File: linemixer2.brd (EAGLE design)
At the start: 101.6 x 58.4 mm, 75 parts, among them IC1 OPA2134P, IC2 OPA2134P, IC3 OPA2134P, IC4 OPA2134P, IC5 OPA2134P, IC6 BUF634P, J1 POWER_JACK

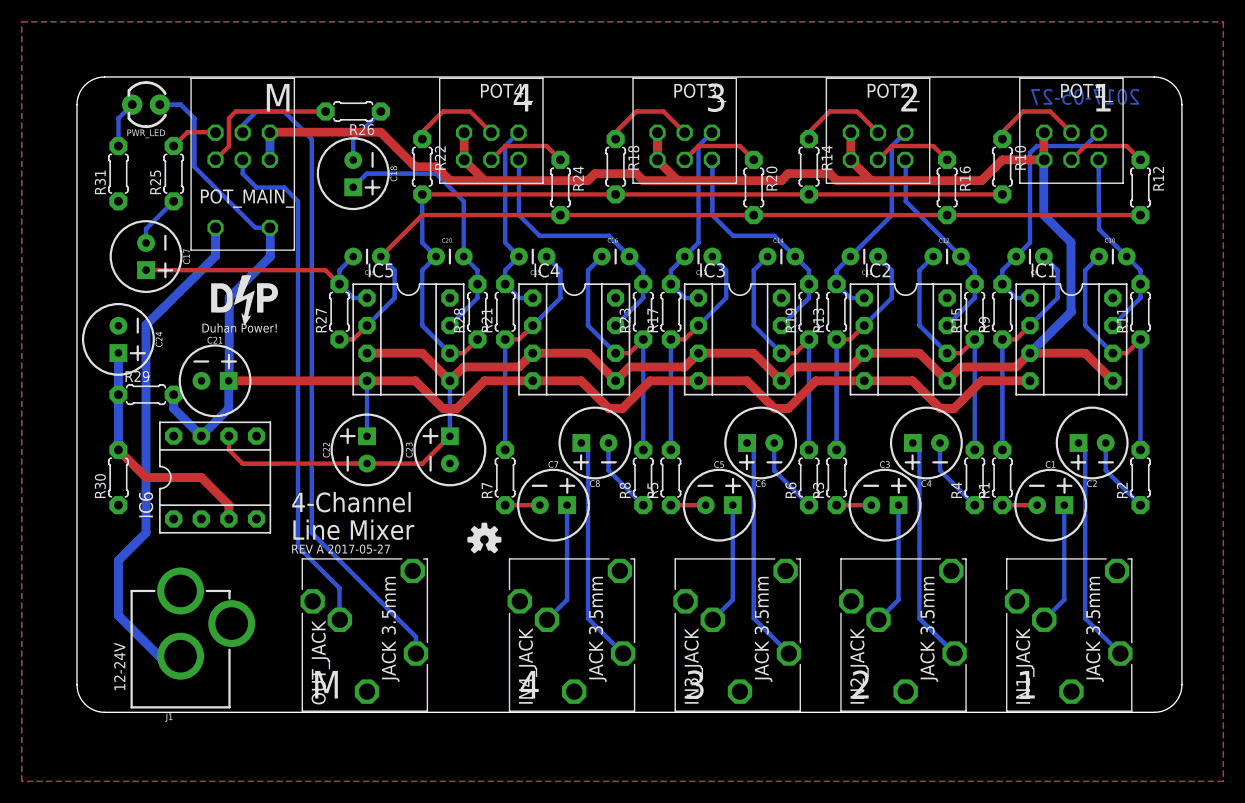
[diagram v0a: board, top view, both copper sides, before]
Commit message: rev b
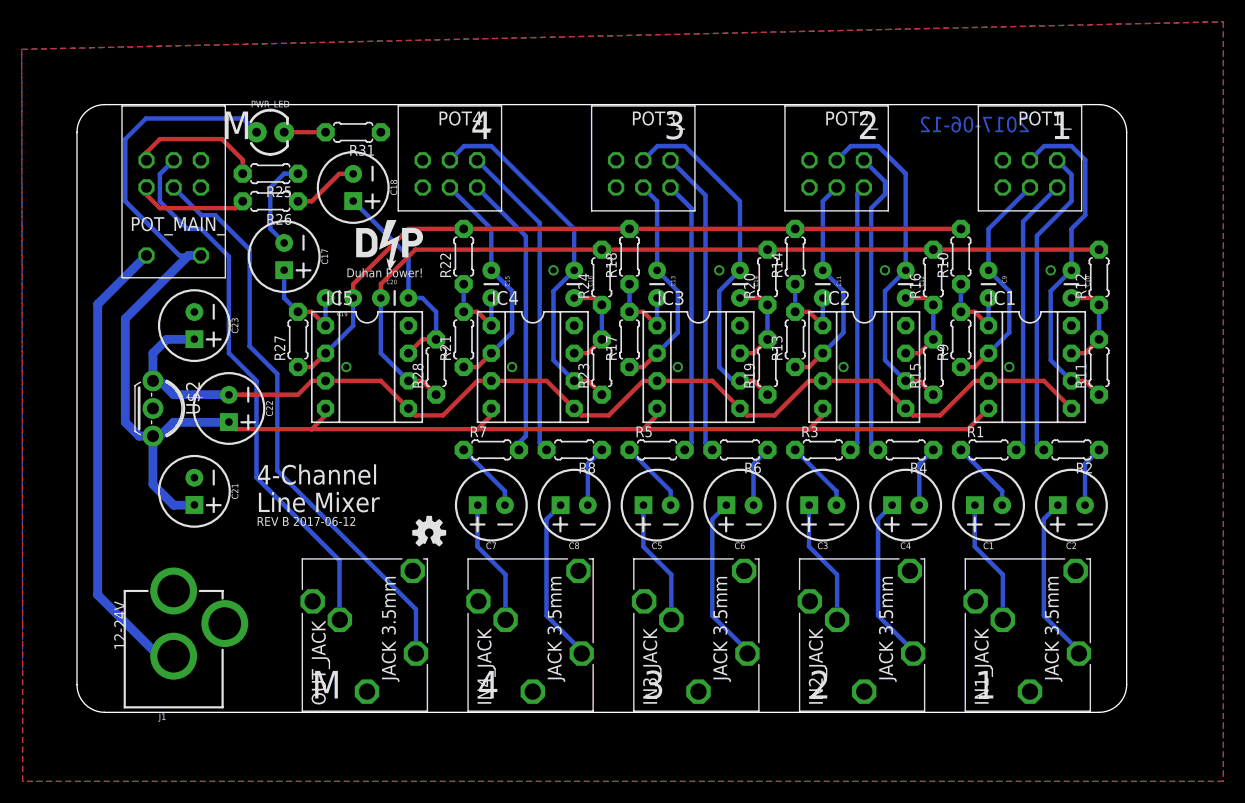
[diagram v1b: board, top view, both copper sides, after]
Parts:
- removed C24: 47u, SparkFun-Capacitors:CPOL-RADIAL-2.5MM-6.5MM
- removed IC6: BUF634P, burr-brown:DIL08
- removed R29, R30: 10k, adafruit:0204/5
- added U$2: TLE2426-TO_92, myparts:TO-92
- R1, R2, R3, R4, R5, R6, R7, R8: value 10k -> 1k
- R10, R12, R14, R16, R18, R20, R22, R24: value 22k -> 1k
- R11, R13, R15, R17, R19, R21, R23, R27, R28, R9: value 47k -> 1k
- R31: value 1k -> 5k
- moved C23 26.1 mm to (10.8, 35.6), turned to 270 degrees
- moved R31 21.9 mm to (25.4, 53.3), turned to 180 degrees
- moved U$1 14.3 mm to (28.6, 43.2)
- moved C22 13.3 mm to (14.0, 27.9), turned to 270 degrees
- moved C17 12.7 mm to (19.1, 41.9)
- moved PWR_LED 11.7 mm to (17.8, 53.3), turned to 0 degrees
- moved R26 11.2 mm to (17.8, 47.0)
- moved C21 10.3 mm to (10.8, 20.3), turned to 270 degrees
- moved R10 9.09 mm to (81.3, 41.9), turned to 90 degrees
- moved R22 9.09 mm to (35.6, 41.9), turned to 90 degrees
- moved R12 9.09 mm to (94.0, 40.0), turned to 90 degrees
- moved R24 9.09 mm to (48.3, 40.0), turned to 90 degrees
- moved R25 8.89 mm to (17.8, 49.5), turned to 180 degrees
- moved R14 8.35 mm to (66.0, 41.9), turned to 90 degrees
- moved R18 8.35 mm to (50.8, 41.9), turned to 90 degrees
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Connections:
- removed net N$19: POT1_.R1-W, R10.1
- removed net N$20: POT2_.R1-W, R14.1
- removed net N$24: POT1_.R2-W, R12.1
- removed net N$26: POT2_.R2-W, R16.1
- removed net N$28: POT3_.R1-W, R18.1
- removed net N$30: POT3_.R2-W, R20.1
- removed net N$32: POT4_.R1-W, R22.1
- removed net N$34: POT4_.R2-W, R24.1
- removed net N$44: C24.1, IC6.3, R29.1, R30.2
- new net N$40: C9.1, IC1.2, POT1_.R2-W, R9.1
- new net N$50: C13.1, IC3.2, POT3_.R2-W, R17.1
- new net N$51: C11.1, IC2.2, POT2_.R2-W, R13.1
- new net N$52: C15.1, IC4.2, POT4_.R2-W, R21.1
- new net N$60: C10.1, IC1.6, POT1_.R1-W, R11.1
- new net N$61: C12.1, IC2.6, POT2_.R1-W, R15.1
- new net N$62: C14.1, IC3.6, POT3_.R1-W, R19.1
- new net N$64: C16.1, IC4.6, POT4_.R1-W, R23.1
- net BUS_L: now also R10.2, R14.2, R18.2, R22.2; no longer R12.2, R16.2, R20.2, R24.2
- net BUS_R: now also R12.2, R16.2, R20.2, R24.2; no longer R10.2, R14.2, R18.2, R22.2
- net GND: now also POT1_.R1-A, POT1_.R2-A, POT2_.R1-A, POT2_.R2-A, POT3_.R1-A, POT3_.R2-A, POT4_.R1-A, POT4_.R2-A, POT_MAIN_.R1-A, POT_MAIN_.R2-A, U$2.PAD2; no longer C24.2, IC6.1, IC6.4, R30.1
- net IN1_L: now also POT1_.R2-B, R1.2; no longer C10.1, IC1.6, R11.1, R2.2
- net IN1_R: now also POT1_.R1-B, R2.2; no longer C9.1, IC1.2, R1.2, R9.1
- net IN2_L: now also POT2_.R2-B, R3.2; no longer C12.1, IC2.6, R15.1, R4.2
- net IN2_R: now also POT2_.R1-B, R4.2; no longer C11.1, IC2.2, R13.1, R3.2
- net IN3_L: now also POT3_.R2-B, R5.2; no longer C14.1, IC3.6, R19.1, R6.2
- net IN3_R: now also POT3_.R1-B, R6.2; no longer C13.1, IC3.2, R17.1, R5.2
- net IN4_L: now also POT4_.R2-B, R7.2; no longer C16.1, IC4.6, R23.1, R8.2
- net IN4_R: now also POT4_.R1-B, R8.2; no longer C15.1, IC4.2, R21.1, R7.2
- net N$17: now also R10.1; no longer POT1_.R1-B
- net N$18: now also R14.1; no longer POT2_.R1-B
- net N$21: now also R12.1; no longer POT1_.R2-B
- net N$25: now also R16.1; no longer POT2_.R2-B
- net N$27: now also R18.1; no longer POT3_.R1-B
- net N$29: now also R20.1; no longer POT3_.R2-B
- net N$31: now also R22.1; no longer POT4_.R1-B
- net N$33: now also R24.1; no longer POT4_.R2-B
- net OUT_L: now also POT_MAIN_.R1-W; no longer POT_MAIN_.R2-W
- net OUT_R: now also POT_MAIN_.R2-W; no longer POT_MAIN_.R1-W
- net VCC: now also U$2.PAD3; no longer IC6.7, R29.2
- net VGND: now also U$2.PAD1; no longer IC6.6, POT1_.R1-A, POT1_.R2-A, POT2_.R1-A, POT2_.R2-A, POT3_.R1-A, POT3_.R2-A, POT4_.R1-A, POT4_.R2-A, POT_MAIN_.R1-A, POT_MAIN_.R2-A
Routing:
- net VGND: track 222.2 -> 104.0 mm, vias 0 -> 1
- net N$64: track 0.00 -> 33.7 mm
- net N$62: track 0.00 -> 33.1 mm
- net N$61: track 0.00 -> 31.6 mm
- net N$60: track 0.00 -> 31.6 mm
- net N$44: track 22.4 -> 0.00 mm
- net N$52: track 0.00 -> 21.5 mm
- net N$40: track 0.00 -> 21.5 mm
- net N$50: track 0.00 -> 20.4 mm
- net N$51: track 0.00 -> 20.4 mm
- net VCC: track 131.3 -> 147.3 mm
- net N$33: track 24.8 -> 9.04 mm
- net N$17: track 23.3 -> 8.15 mm
- net N$22: track 24.4 -> 9.96 mm
- net BUS_L: track 82.4 -> 68.5 mm
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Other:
- board size 101.6 x 58.4 mm -> 96.5 x 55.9 mm
- board text added: "2017-06-12"
- board text added: "REV B 2017-06-12"
- board text removed: "2017-05-27"
- board text removed: "REV A 2017-05-27"
